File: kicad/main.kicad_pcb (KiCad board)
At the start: 2 copper layers, 200 x 100 mm, 48 parts, among them J1 Barrel_Jack, J2 UART, P1 Mini-DIN_6pins_ver3, SW1 Reset, SW2 SW_Push_DPDT, U1 KM1810VM88, U10 L7805, U11 15 MHz, U12 8255, U13 uSD adapter, U14 8259, U15 AS6C4008-55PCN, U16 16550, U17 T6963C, U18 1.8432 MHz, U19 ATF16V8, U2 W27C512, U3 AS6C4008-55PCN, U4 74HC573, U5 74HC573, U6 ATF16V8, U7 DS1813-5+, U8 74HC14, U9 8253

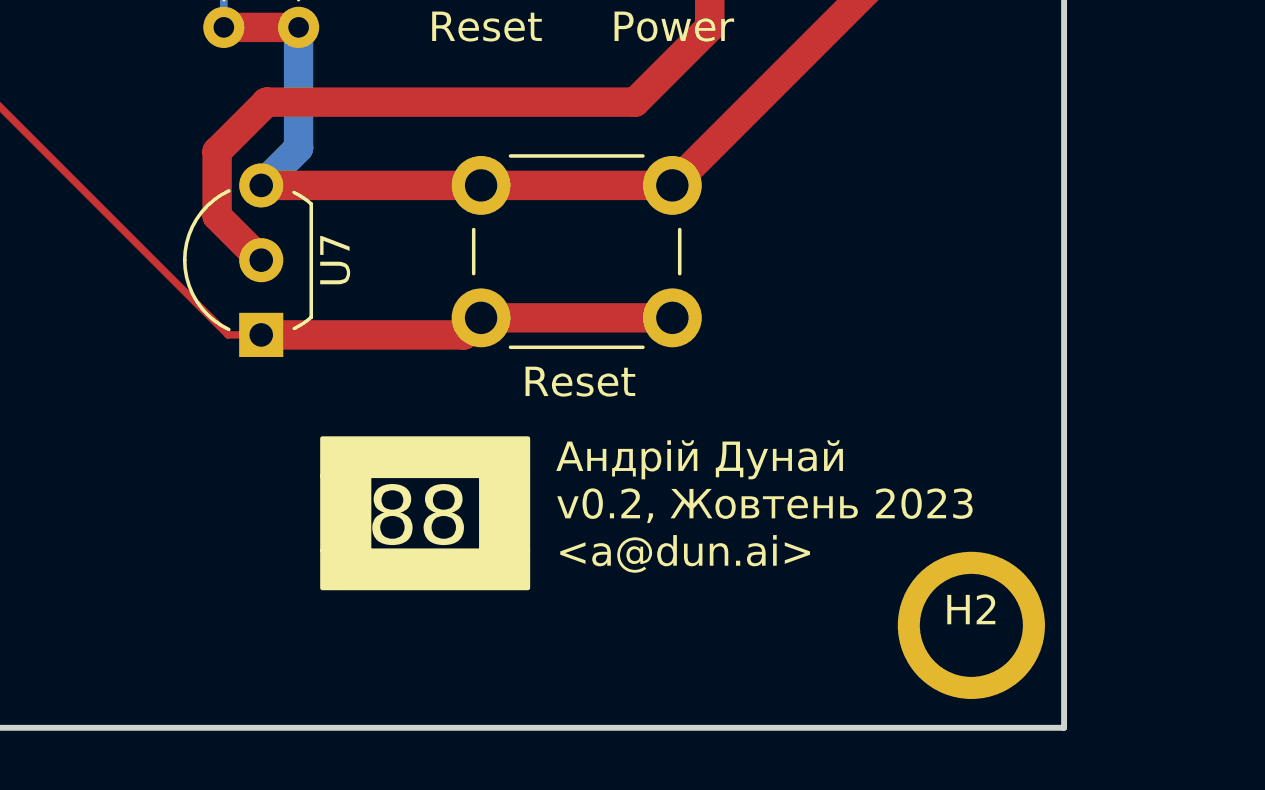
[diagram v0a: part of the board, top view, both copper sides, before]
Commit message: Update logo
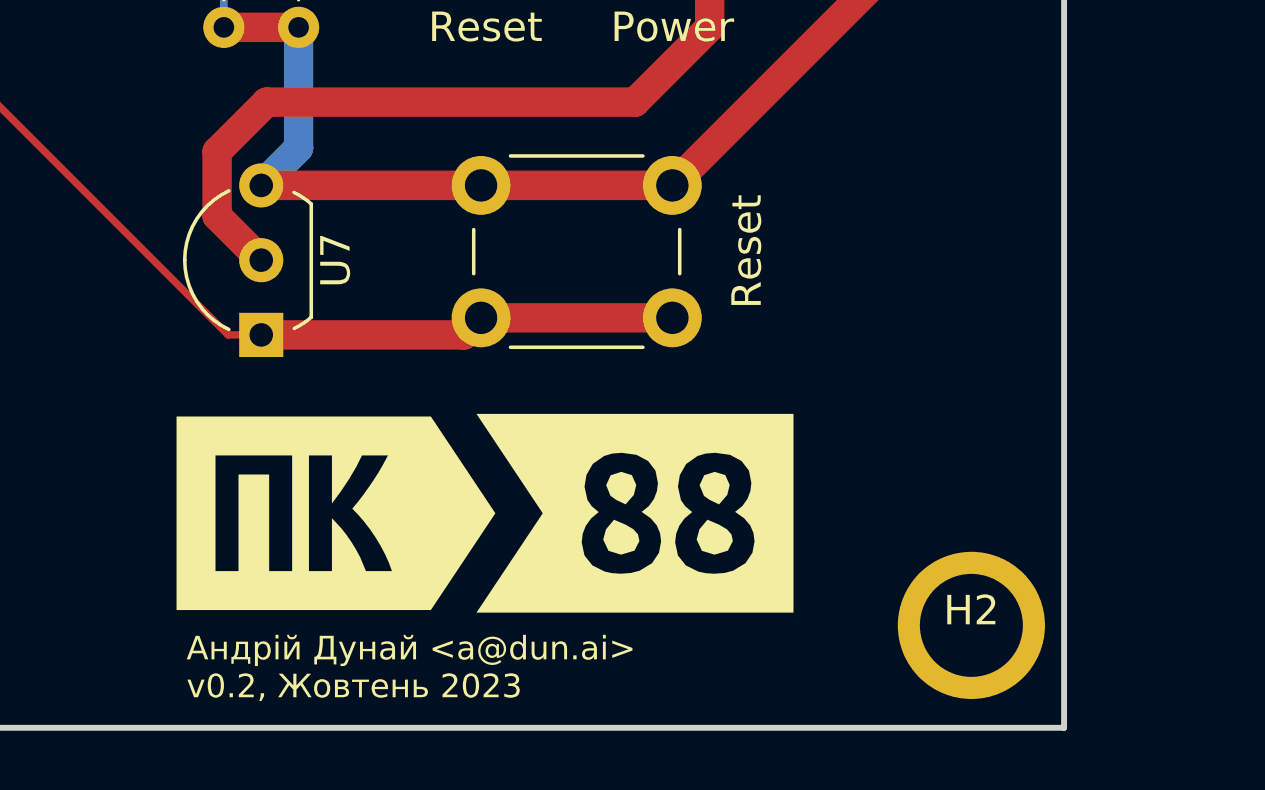
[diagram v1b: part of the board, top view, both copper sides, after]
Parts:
- added kibuzzard-65254FD7: G***, kibuzzard-65254FD7, F.Cu at (195.6, 110.5)
- added kibuzzard-65254FDB: G***, kibuzzard-65254FDB, F.Cu at (205.7, 110.5)
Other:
- board text added: "Андрій Дунай <a@dun.ai> v0.2, Жовтень 2023"
- board text removed: "88"
- board text removed: "Андрій Дунай v0.2, Жовтень 2023 <a@dun.ai>"
